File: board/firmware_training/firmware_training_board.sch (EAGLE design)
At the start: 15 parts, among them J1 GY-521-MPU-6050, SW1 PTS645, SW2 PTS645

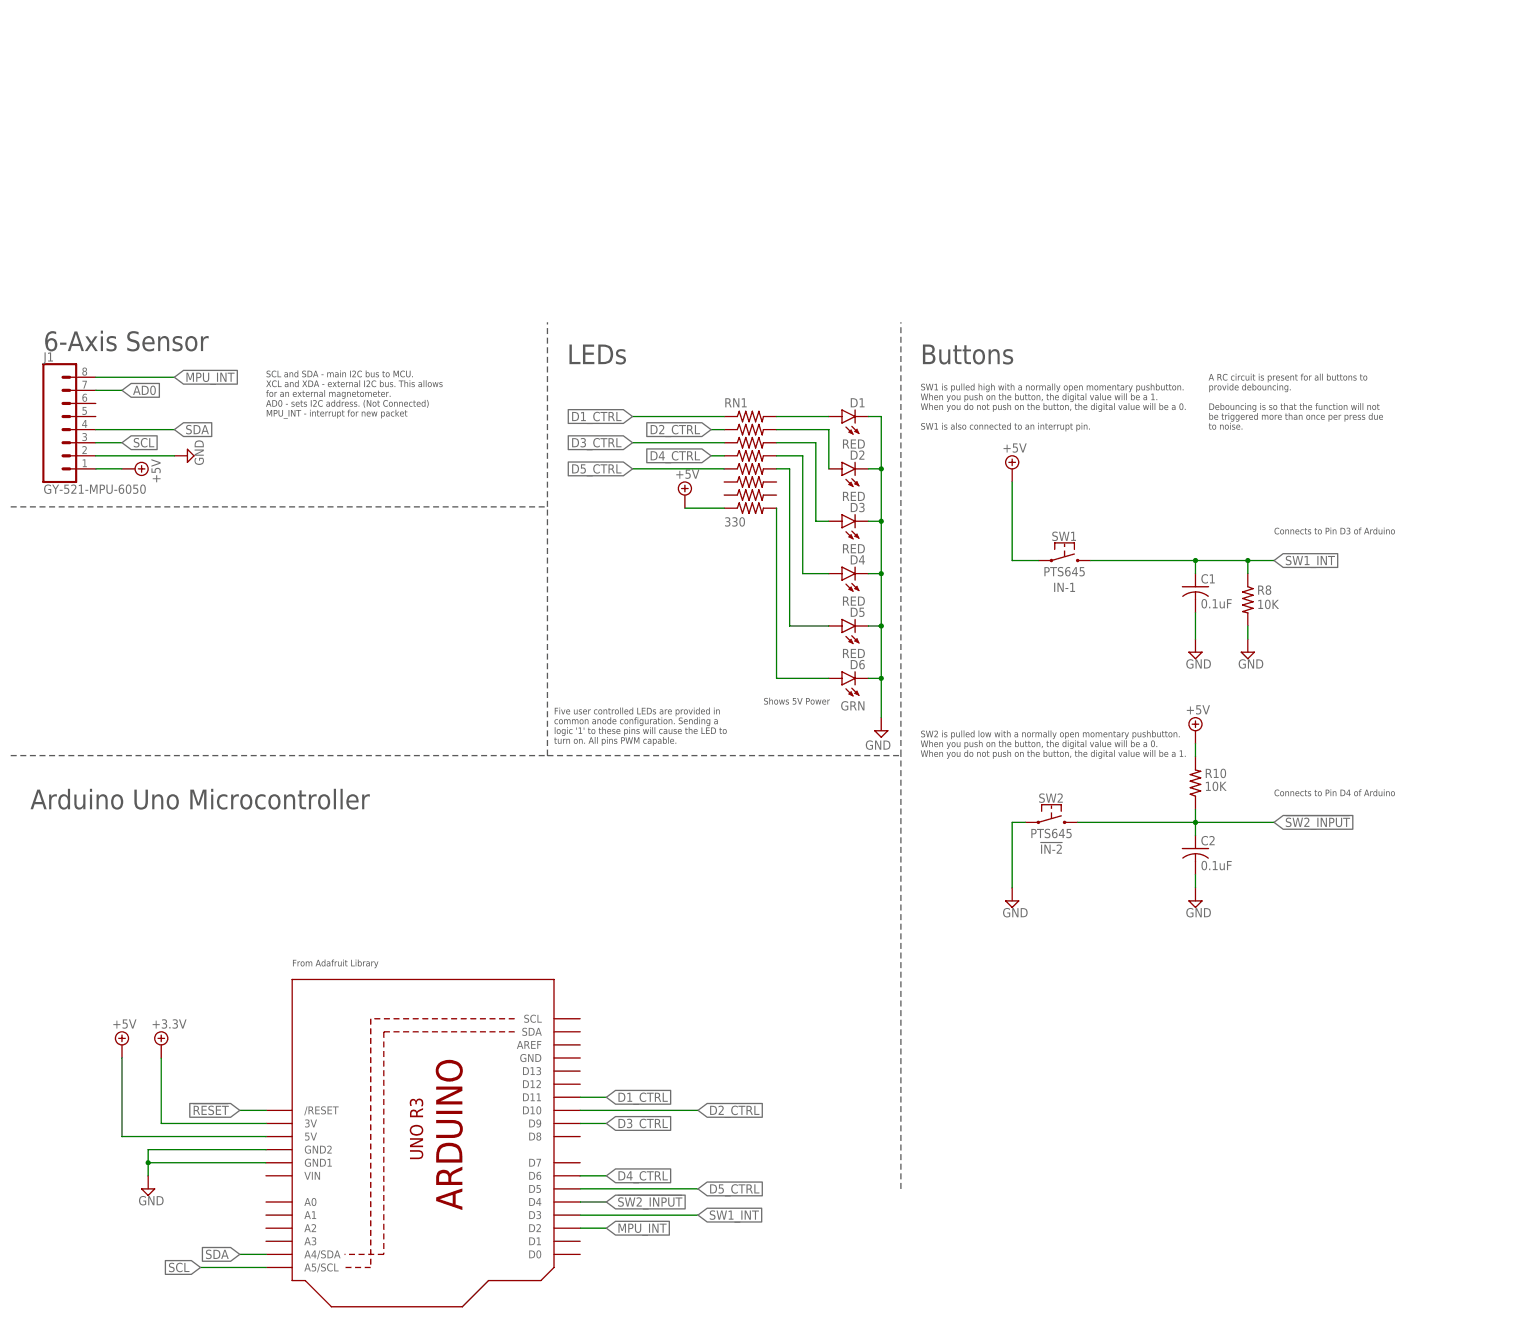
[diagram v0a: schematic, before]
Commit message: Finished schematic, started board
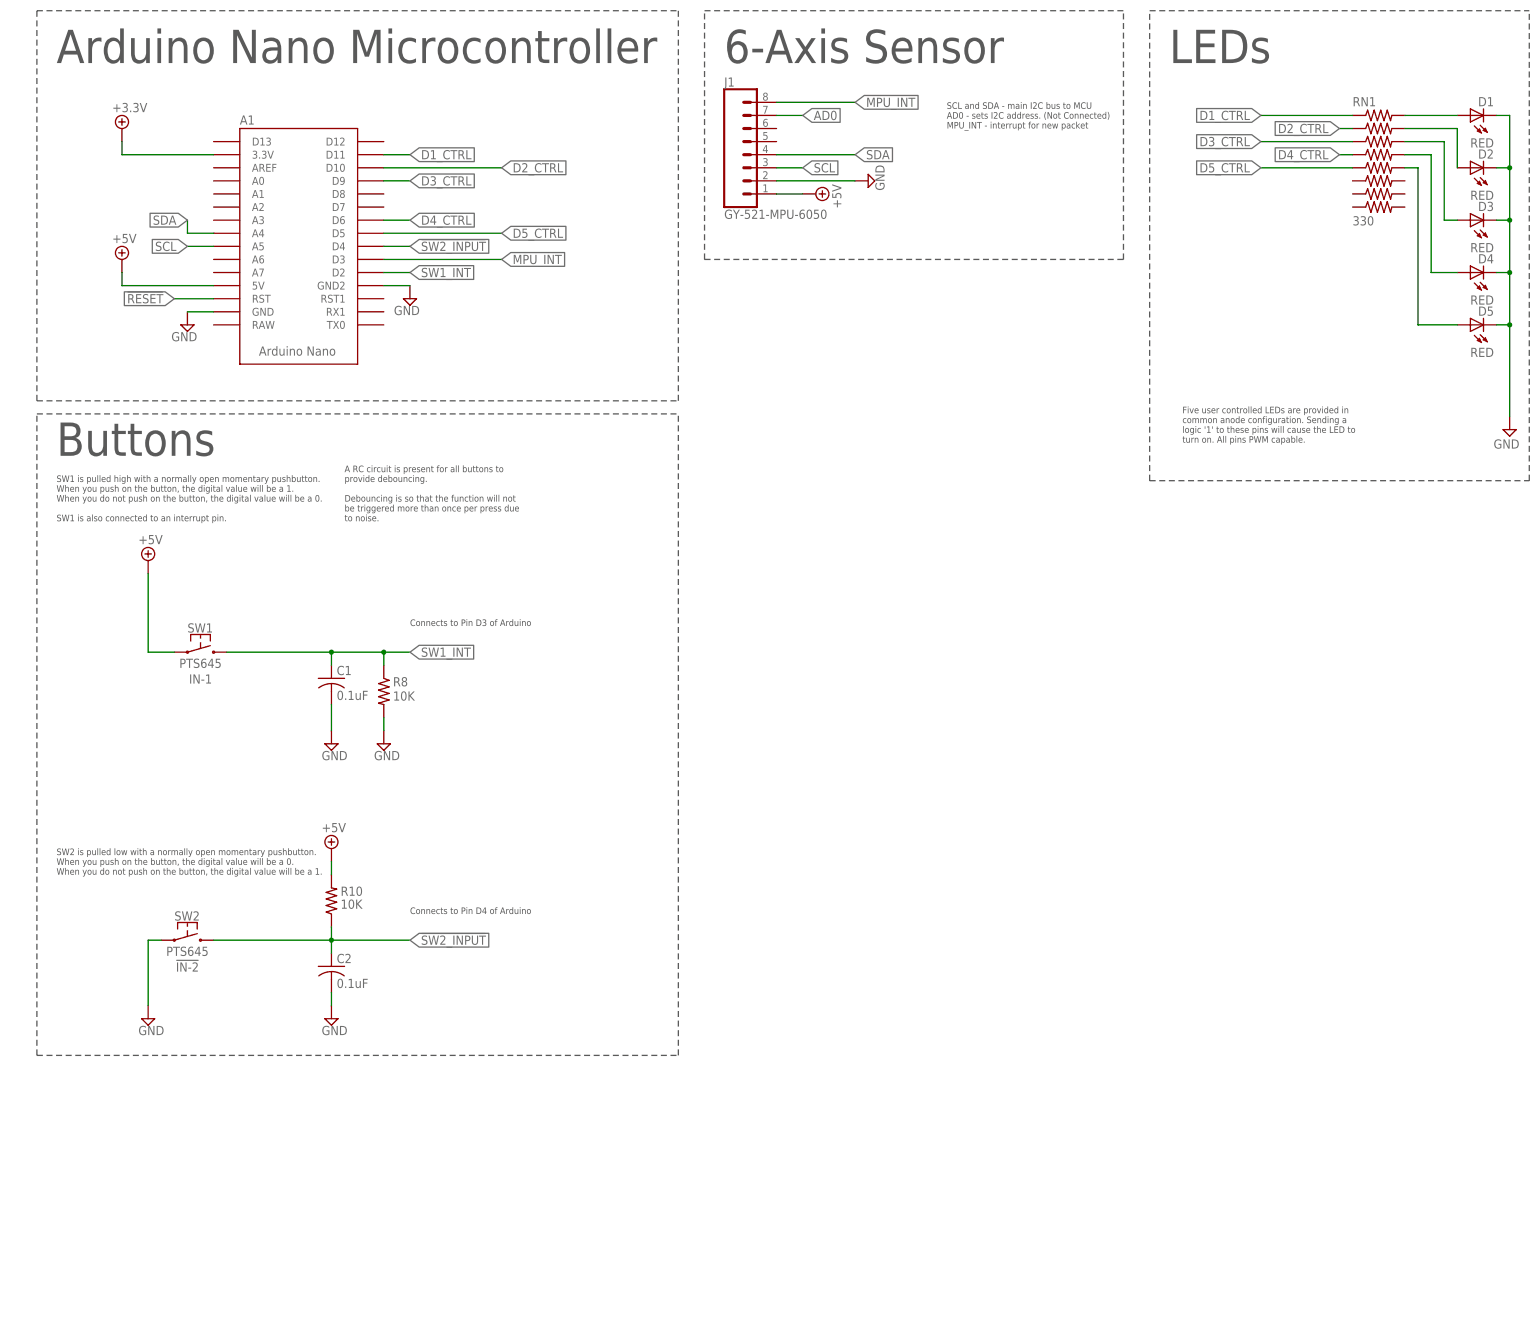
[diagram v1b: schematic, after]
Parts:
- removed D6: GRN, led:LEDCHIP-LED0603
- A1: value ARDUINOR3-NOIOREF-NOTEXT -> NANO; device adafruit:ARDUINOR3-NOIOREF-NOTEXT -> firmware_training_board:NANO
- D1: device led:LEDCHIP-LED0603 -> adafruit:LED5MM
- D2, D3, D4, D5: device led:LEDCHIP-LED0603 -> firmware_training_board:LED5MM
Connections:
- net N$2 renamed D1_LED
- net N$3 renamed D2_LED
- net N$4 renamed D3_LED
- net N$5 renamed D4_LED
- net N$6 renamed D5_LED
- removed net N$9: D6.A, RN1.16
- net !RESET: now also A1.RST; no longer A1./RESET
- net +3.3V: now also A1.3.3V; no longer A1.3V
- net +5V: no longer RN1.15
- net GND: now also A1.GND; no longer A1.GND1, D6.C
- net MPU_INT: now also A1.D3; no longer A1.D2
- net SCL: now also A1.A5; no longer A1.A5/SCL
- net SDA: now also A1.A4; no longer A1.A4/SDA
- net SW1_INT: now also A1.D2; no longer A1.D3
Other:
- note added: "Arduino Nano Microcontroller"
- note added: "SCL and SDA - main I2C bus to MCU AD0 - sets I2C address. (Not Connected) MPU_INT - interrupt for new packet"
- note removed: "Arduino Uno Microcontroller"
- note removed: "From Adafruit Library"
- note removed: "SCL and SDA - main I2C bus to MCU. XCL and XDA - external I2C bus. This allows for an external magnetometer. AD0 - sets I2C address. (Not Connected) MPU_INT - interrupt for new packet"
- note removed: "Shows 5V Power"
- moved on the sheet: C1, C2, J1, R10, R8, RN1, SW1, SW2
